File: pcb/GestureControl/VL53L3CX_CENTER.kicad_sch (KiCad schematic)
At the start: 52 parts, among them J13 690367291076, J14 690367291076, J15 690367291076, J16 690367291076, J20 690367291076, J21 690367291076, U3 VL53L3CXV0DH_1, U4 VL53L3CXV0DH_1, U5 VL53L3CXV0DH_1, U8 VL53L3CXV0DH_1

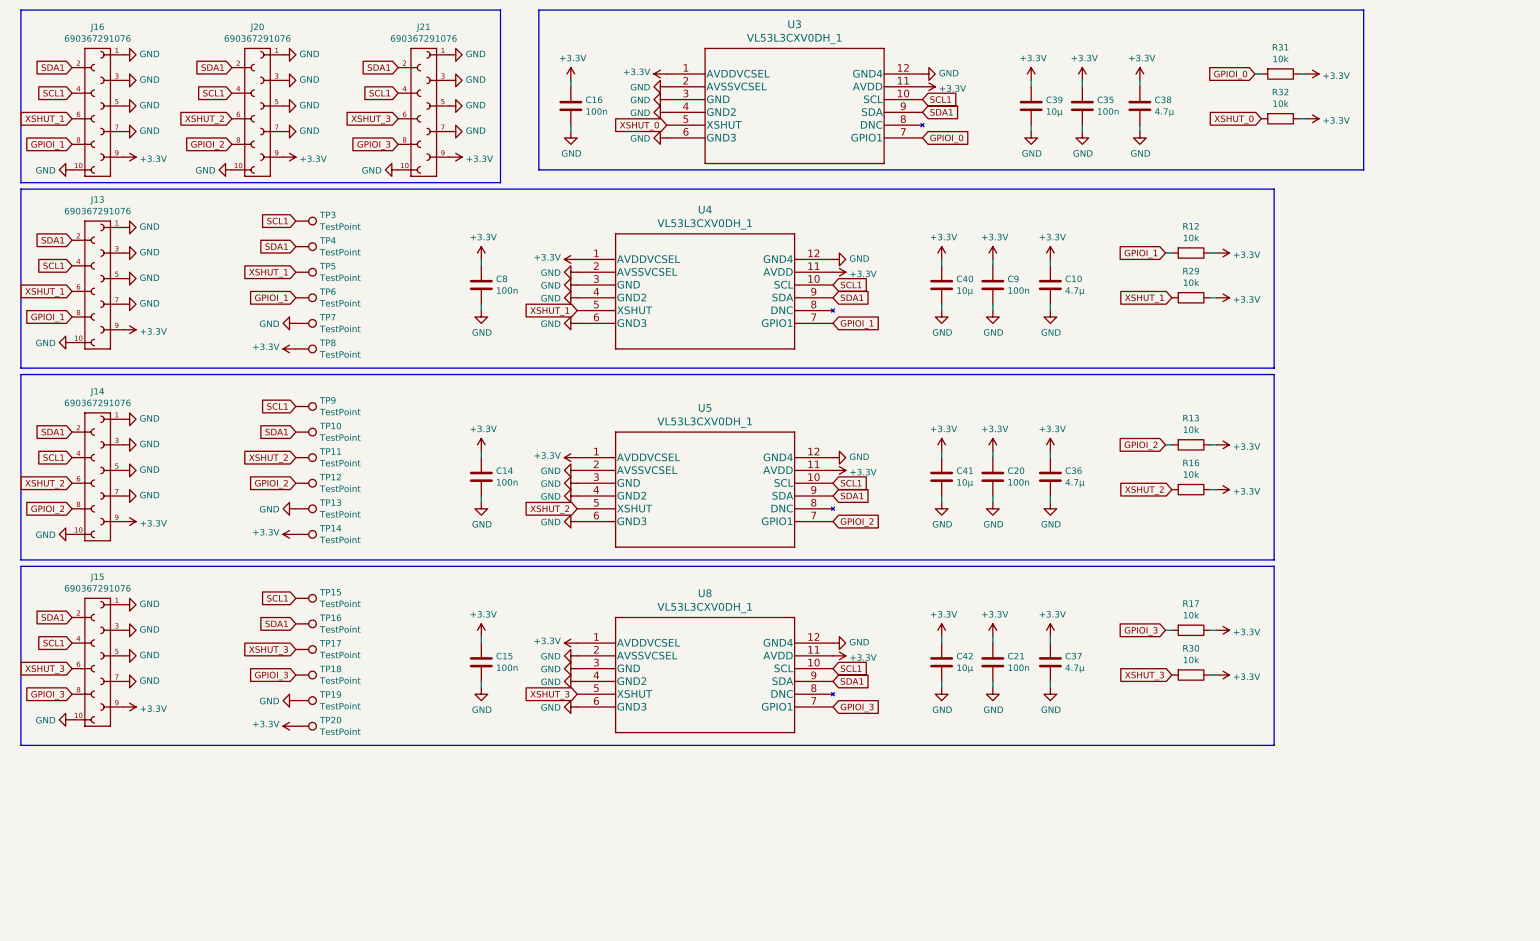
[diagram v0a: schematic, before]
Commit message: add breakoutboard
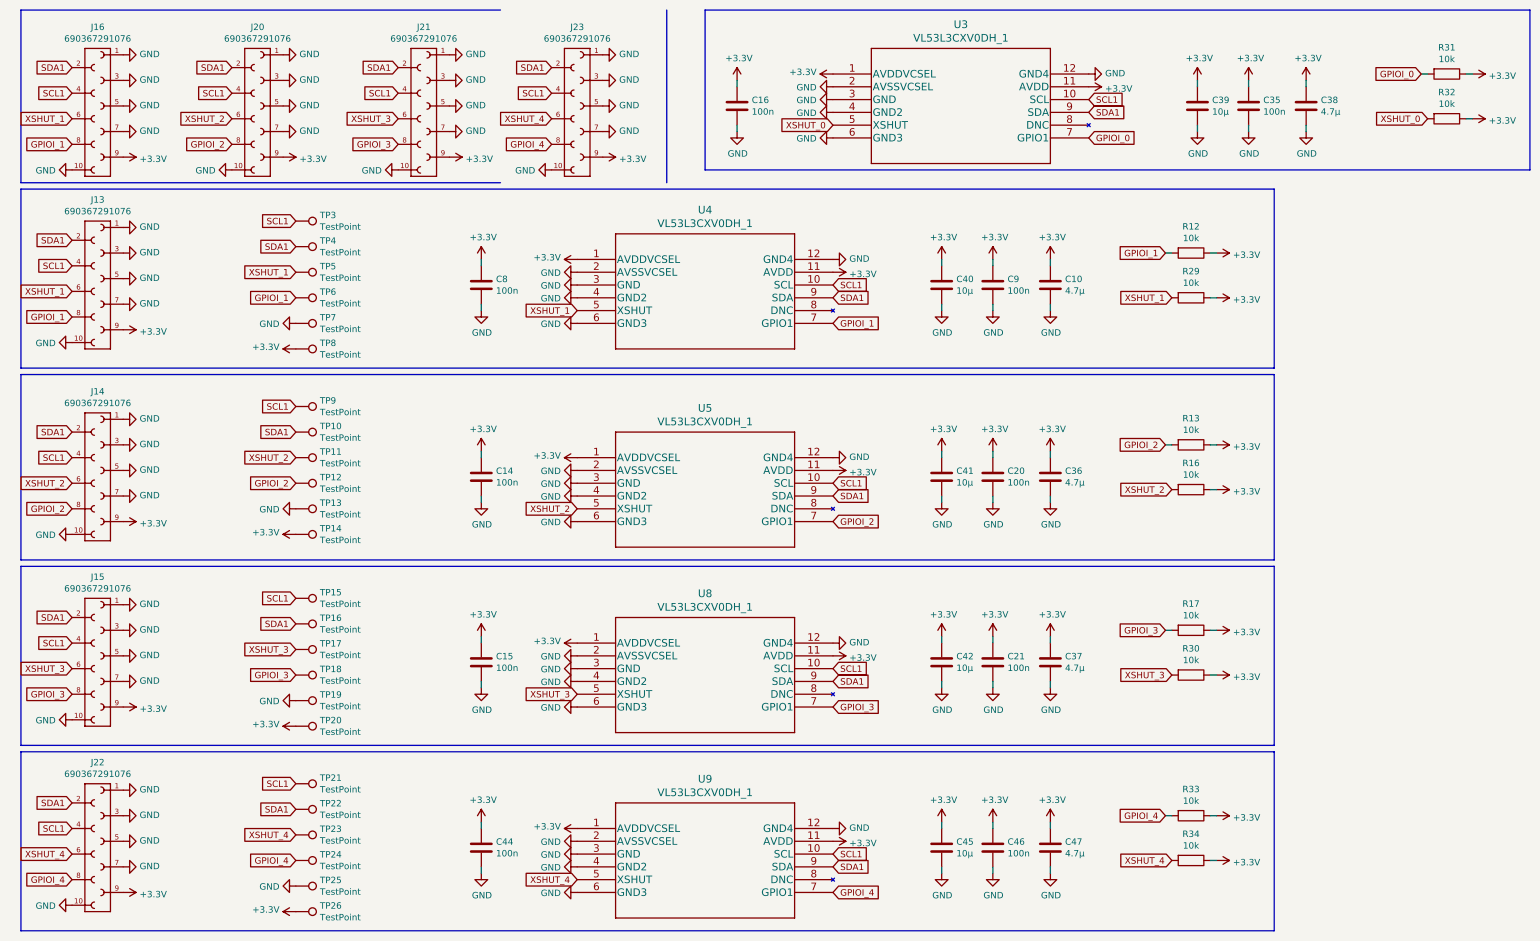
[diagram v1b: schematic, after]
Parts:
- added C44, C46: 100n, Capacitor_SMD:C_0603_1608Metric_Pad1.08x0.95mm_HandSolder, symbol Device:C
- added C45: 10µ, Capacitor_SMD:C_1206_3216Metric_Pad1.33x1.80mm_HandSolder, symbol Device:C
- added C47: 4.7µ, Capacitor_SMD:C_0805_2012Metric_Pad1.18x1.45mm_HandSolder, symbol Device:C
- added J22, J23: 690367291076, WR-MM Female SMT Connector:WR-MM_Female_SMT_Connector, symbol WR-MM_Female_SMT_Connector:690367291076
- added R33, R34: 10k, Resistor_SMD:R_0805_2012Metric_Pad1.20x1.40mm_HandSolder, symbol Device:R
- added TP21, TP22, TP23, TP24, TP25, TP26: TestPoint, TestPoint:TestPoint_Pad_D2.0mm, symbol Connector:TestPoint
- added U9: VL53L3CXV0DH_1, VL53L3CX:VL53L3CXV0DH&slash_1, symbol VL53L3CX:VL53L3CXV0DH_1
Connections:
- net +3V3: now also C44.1, C45.1, C46.1, C47.1, J22.9, J23.9, R33.1, R34.1, TP26.1, U9.1 (AVDDVCSEL), U9.11 (AVDD)
- net GND: now also C44.2, C45.2, C46.2, C47.2, J22.1, J22.10, J22.3, J22.5, J22.7, J23.1, J23.10, J23.3, J23.5, J23.7, TP25.1, U9.12 (GND4), U9.2 (AVSSVCSEL), U9.3 (GND), U9.4 (GND2), U9.6 (GND3)
- net SCL1: now also J22.4, J23.4, TP21.1, U9.10 (SCL)
- net SDA1: now also J22.2, J23.2, TP22.1, U9.9 (SDA)
- new net GPIOI_4: J22.8, J23.8, R33.2, TP24.1, U9.7 (GPIO1)
- new net XSHUT_4: J22.6, J23.6, R34.2, TP23.1, U9.5 (XSHUT)
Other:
- moved on the sheet: C16, C35, C38, C39, R31, R32, U3
